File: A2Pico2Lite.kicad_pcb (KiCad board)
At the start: 2 copper layers, 65.5 x 44.1 mm, 63 parts, among them J1 PinHeader_1x03_P2.54mm_Vertic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, J2 SolderJumper-2_P1.3mm_Bridged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, U1 Pico

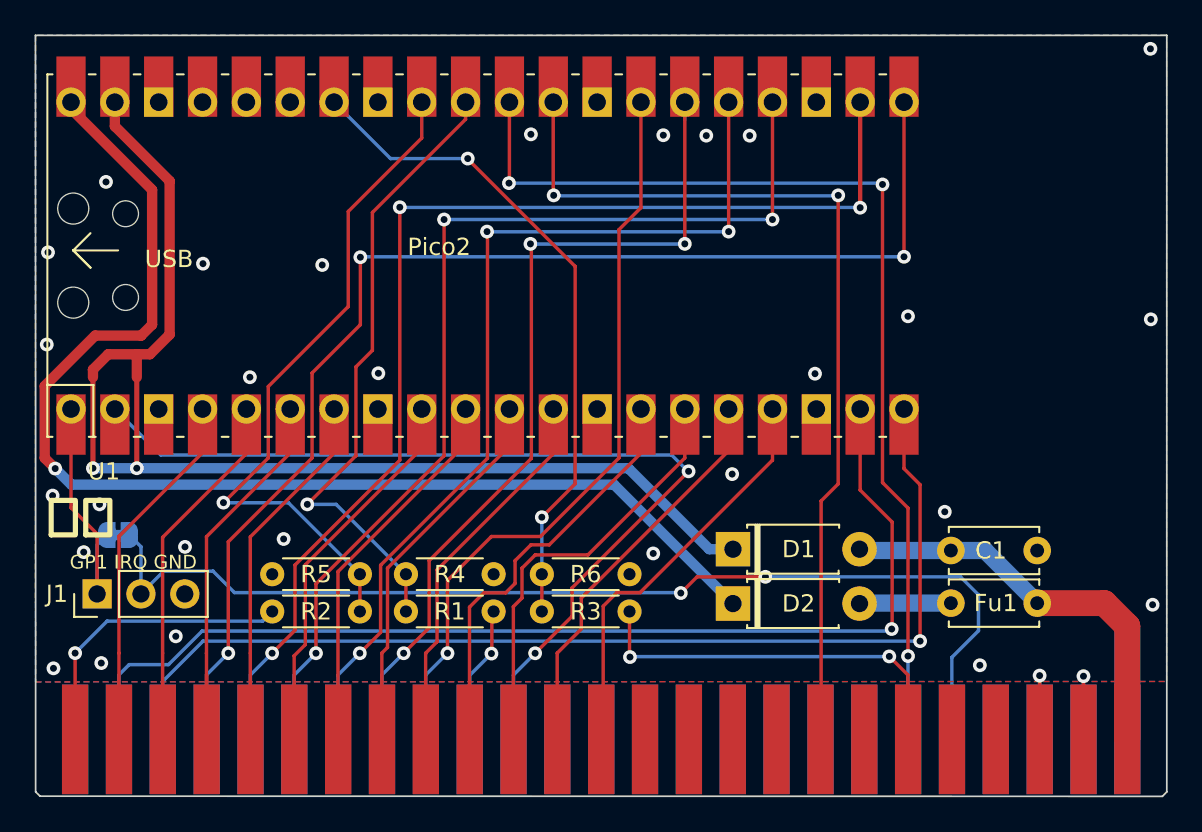
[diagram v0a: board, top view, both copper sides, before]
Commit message: Add files via upload
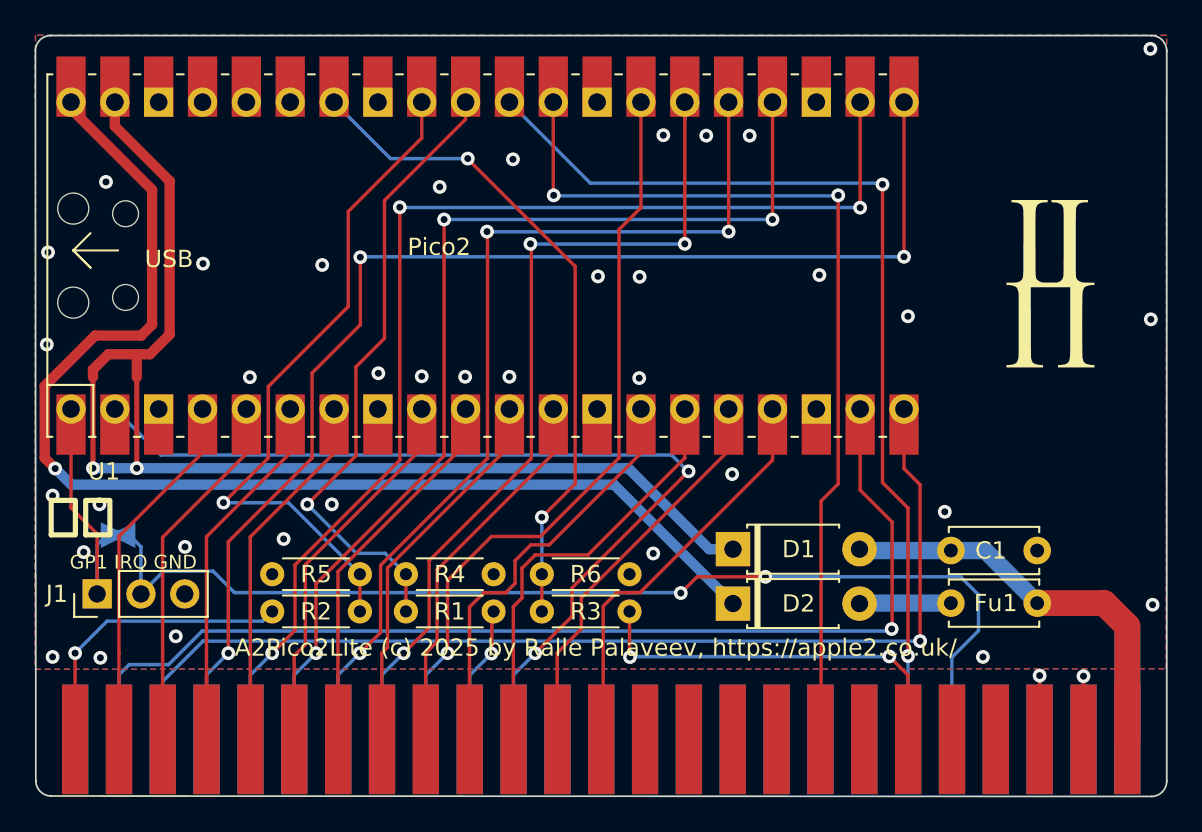
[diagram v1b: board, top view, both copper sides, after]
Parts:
- added G***: LOGO, LOGO, F.Cu at (174.1, 97.5)
- added REF**: OSHW-Logo2_7.3x6mm_SilkScreen, Symbol:OSHW-Logo2_7.3x6mm_SilkScreen, B.Cu at (174.0, 98.0)
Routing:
- net ~{Reset}: track 59.3 -> 56.5 mm, vias 3 -> 2
- net GND: vias 28 -> 36
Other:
- outline, holes or cut-outs redrawn
- board text added: "A2Pico2Lite (c) 2025 by Ralle Palaveev, https://apple2.co.uk/"
